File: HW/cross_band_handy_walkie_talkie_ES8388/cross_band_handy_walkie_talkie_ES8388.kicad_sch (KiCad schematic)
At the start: 91 parts, among them J1 USB_C_Receptacle, J2 Micro_SD_Card_Det, J9 Conn_01x04, Q1 nMOS, Q2 AO3401A, Q3 AO3401A, Q4 AO3401A, SW1 MCU_RESET, SW2 MCU_RESET, U1 SRV05-4, U2 ESP32-S3-WROOM-1, U3 AMS1117-3.3, U4 TP5000

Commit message: r
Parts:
- added BT2: Battery_Cell, Connector_JST:JST_XH_B2B-XH-AM_1x02_P2.50mm_Vertical, symbol Device:Battery_Cell
- added R24: 10, Resistor_SMD:R_0402_1005Metric, symbol Device:R_Small
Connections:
- net AMP_L: now also R49.1; no longer R48.1
- net G1: now also R48.1; no longer R49.1
- net GND: now also BT2.2 (-)
- net GPIO_18: now also R24.2
- net at BT1.1 (+), C10.1, C11.1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: now also BT2.1 (+)
- new net PTT3: R24.1
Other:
- moved on the sheet: BT1, C16, C17

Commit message: y
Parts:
- added D8: red, LED_SMD:LED_0603_1608Metric, symbol Device:LED_Small
- added J10: Conn_01x04, Connector_PinHeader_2.54mm:PinHeader_1x03_P2.54mm_Vertical, symbol Connector_Generic:Conn_01x04
- added R45: 1k, Resistor_SMD:R_0603_1608Metric, symbol Device:R
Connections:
- net GND: now also D8.2 (A), J10.1 (Pin_1)
- net GPIO_43: now also J10.3 (Pin_3)
- net GPIO_44: now also J10.2 (Pin_2)
- net +BATT: now reaches BT1.1 (+), BT2.1 (+), C10.1, C11.1, C16.1, C17.2, L1.1, R43.1, U4.9 (BAT)
- net +BATT: now also R45.2
- new net: D8.1 (K), R45.1
- no-connect marks 14 -> 16
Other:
- note added: "COMMON RF POWER SET PIN"
- note added: "EXTERNAL PTT PIN"
- note added: "MODULE 1"
- note added: "MODULE 2"
- note added: "POWER AMPLIFIER"
- note added: "POWER SUPPLY: BMS + CHARGEING + REGULATION"
- note added: "RF MODULE PIN SETUP"
- note added: "reversed on purpose"
- title: (none) -> Cross band handy walkie talkie V2
- moved on the sheet: BT1, BT2, C10, C11, C12, C13, C16, C17, C53, C57, C58, C59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

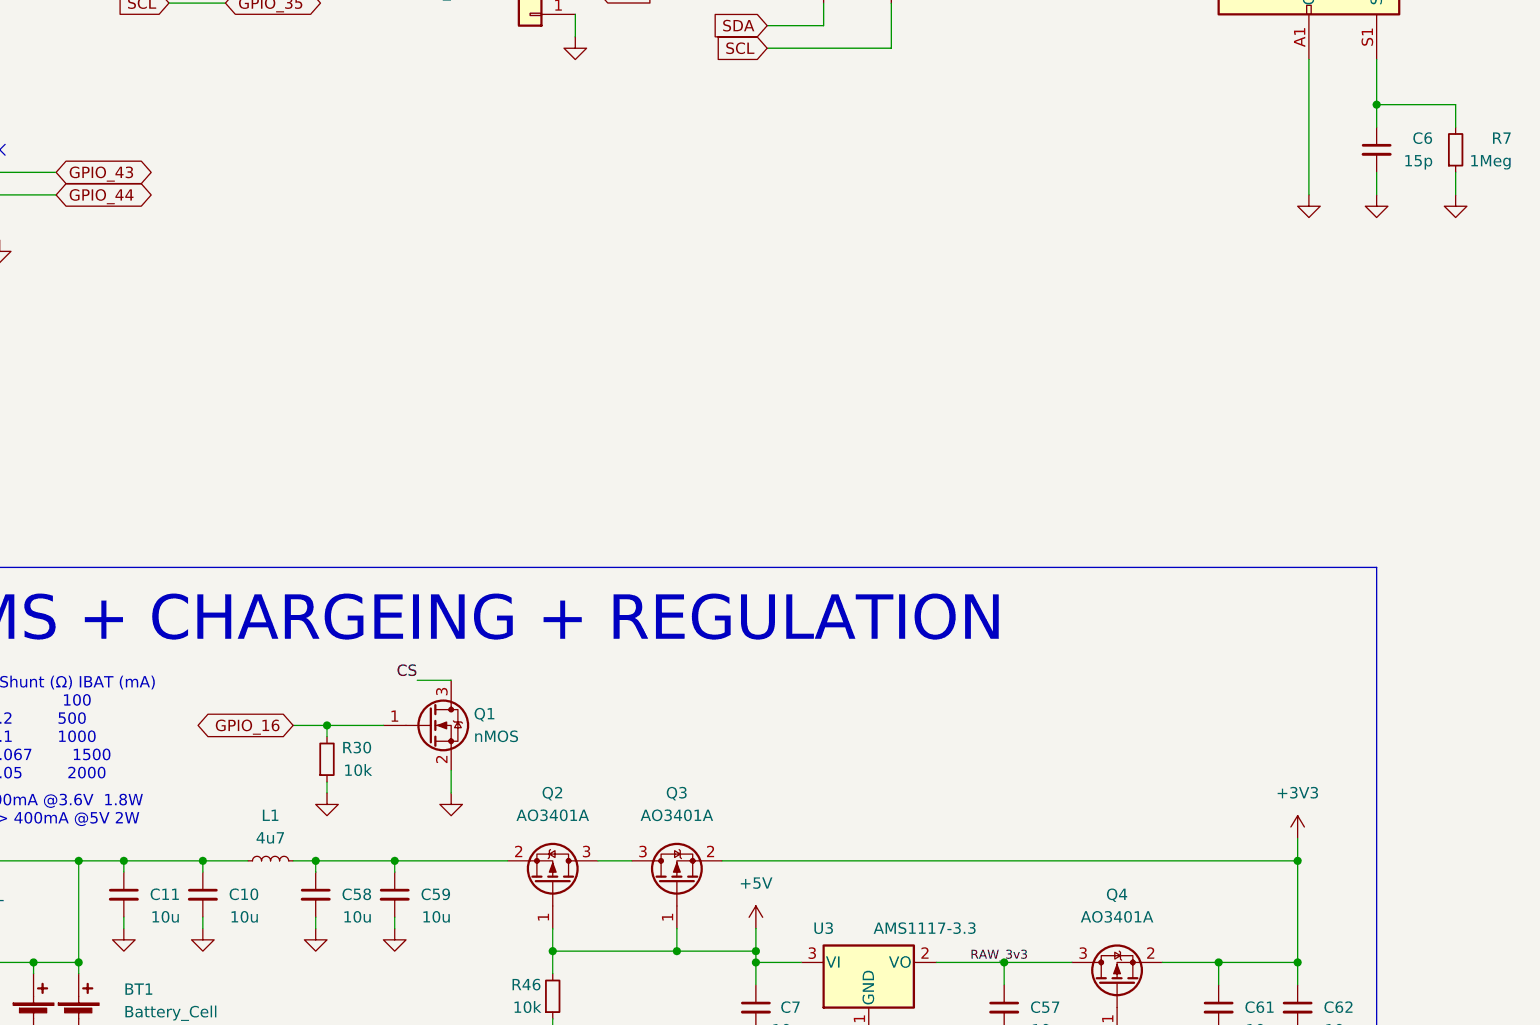
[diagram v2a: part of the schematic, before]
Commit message: b
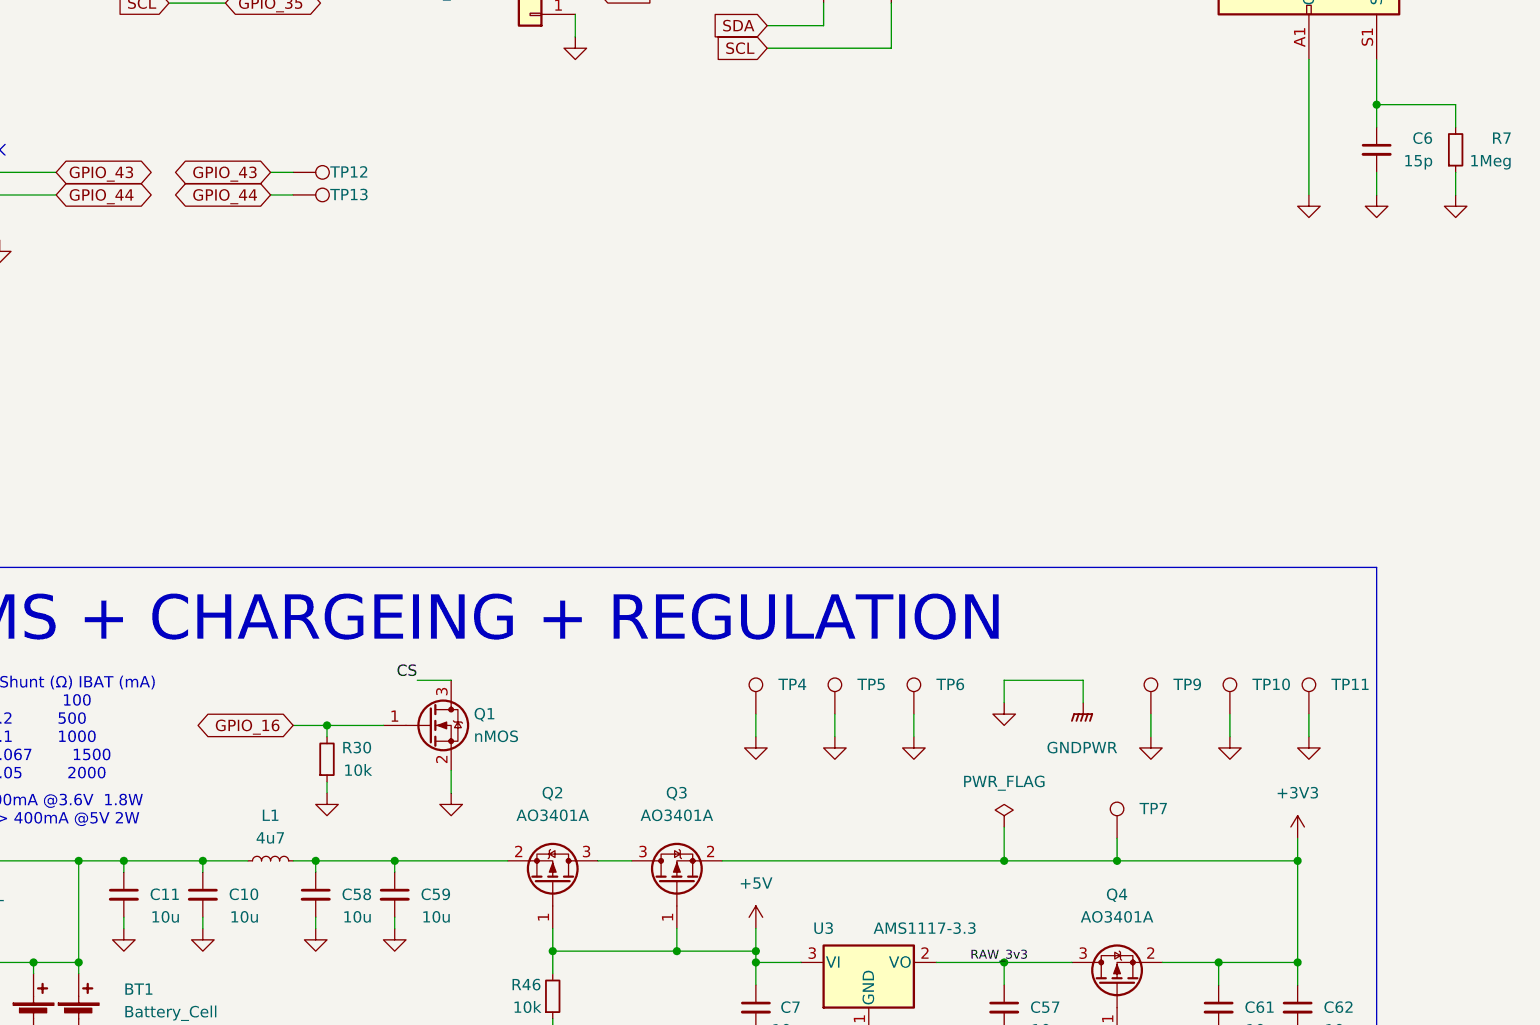
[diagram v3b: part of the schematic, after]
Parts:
- added TP10, TP11, TP12, TP13, TP4, TP5, TP6, TP7, TP9: TestPoint, TestPoint:TestPoint_Pad_1.0x1.0mm, symbol Connector:TestPoint
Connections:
- net +3V3: now also TP7.1
- net GND: now also TP10.1, TP11.1, TP4.1, TP5.1, TP6.1, TP9.1
- net GPIO_43: now also TP12.1
- net GPIO_44: now also TP13.1
